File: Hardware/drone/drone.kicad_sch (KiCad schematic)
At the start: 11 parts, among them M1 Motor_DC, M2 Motor_DC, M3 Motor_DC, M4 Motor_DC, U1 ESP32-DEVKITC, U2 MPU6050 DevKit, U3 HW_611, U4 DRV8833, U5 DRV8833, U6 MT3608

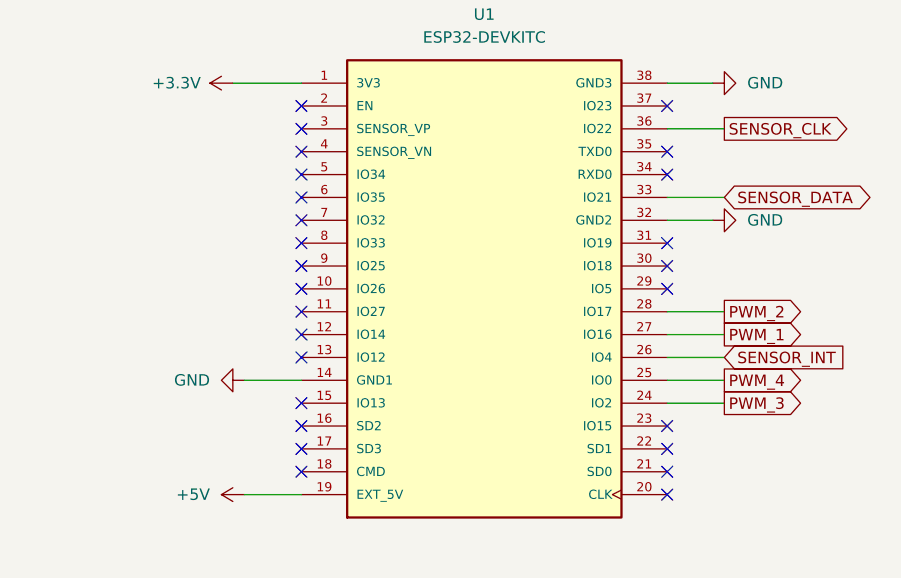
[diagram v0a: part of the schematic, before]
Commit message: PCB design v1.0
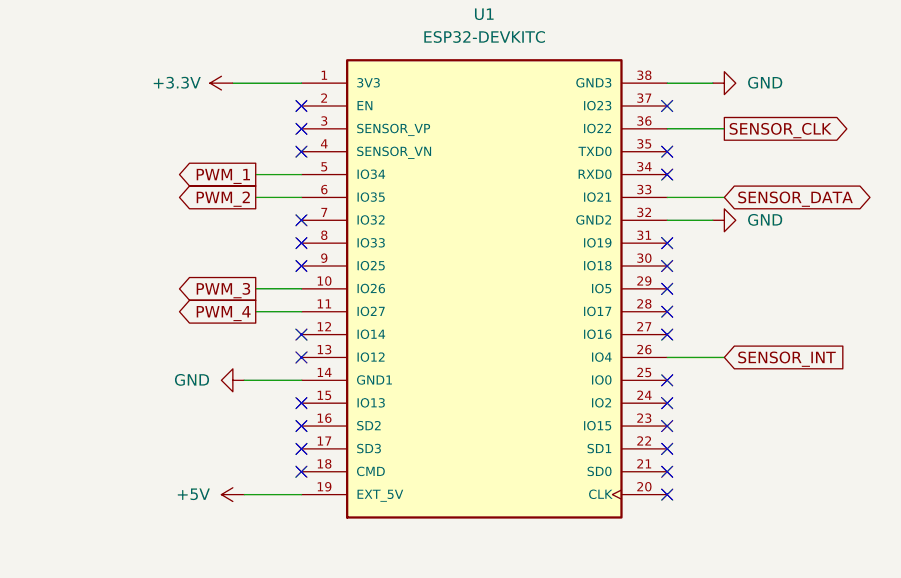
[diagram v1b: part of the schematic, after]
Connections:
- net PWM_1: now also U1.5 (IO34); no longer U1.27 (IO16)
- net PWM_2: now also U1.6 (IO35); no longer U1.28 (IO17)
- net PWM_3: now also U1.10 (IO26); no longer U1.24 (IO2)
- net PWM_4: now also U1.11 (IO27); no longer U1.25 (IO0)
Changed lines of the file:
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@@
+	)
+	(no_connect
+		(at 215.9 121.92)
 	)
 	(no_connect
@@
 	)
 	(no_connect
+		(at 215.9 119.38)
+	)
+	(no_connect
 		(at 128.27 48.26)
 	)
@@
 	)
 	(no_connect
-		(at 175.26 99.06)
-	)
-	(no_connect
 		(at 175.26 104.14)
 	)
 	(no_connect
-		(at 175.26 111.76)
-	)
-	(no_connect
 		(at 67.31 44.45)
 	)
 	(no_connect
+		(at 215.9 111.76)
+	)
+	(no_connect
 		(at 215.9 88.9)
 	)
@@
 	)
 	(no_connect
-		(at 175.26 109.22)
-	)
-	(no_connect
 		(at 175.26 93.98)
 	)
@@
 	)
 	(no_connect
-		(at 175.26 96.52)
+		(at 215.9 114.3)
 	)
 	(no_connect
@@
 	(wire
 		(pts
-			(xy 215.9 119.38) (xy 222.25 119.38)
+			(xy 170.18 99.06) (xy 175.26 99.06)
 		)
 		(stroke
@@
 	(wire
 		(pts
-			(xy 215.9 111.76) (xy 222.25 111.76)
+			(xy 170.18 96.52) (xy 175.26 96.52)
 		)
 		(stroke
@@
 	(wire
 		(pts
+			(xy 170.18 111.76) (xy 175.26 111.76)
+		)
+		(stroke
+			(width 0)
+			(type default)
+		)
+	)
+	(wire
+		(pts
 			(xy 215.9 86.36) (xy 220.98 86.36)
 		)
@@
 	(wire
 		(pts
+			(xy 170.18 109.22) (xy 175.26 109.22)
+		)
+		(stroke
+			(width 0)
+			(type default)
+		)
+	)
+	(wire
+		(pts
 			(xy 67.31 36.83) (xy 72.39 36.83)
 		)
@@
 	(wire
 		(pts
-			(xy 215.9 121.92) (xy 222.25 121.92)
-		)
-		(stroke
-			(width 0)
-			(type default)
-		)
-	)
-	(wire
-		(pts
-			(xy 215.9 114.3) (xy 222.25 114.3)
-		)
-		(stroke
-			(width 0)
-			(type default)
-		)
-	)
-	(wire
-		(pts
 			(xy 168.91 132.08) (xy 175.26 132.08)
 		)
@@
 		)
 	)
+	(global_label "PWM_4"
+		(shape output)
+		(at 170.18 111.76 180)
+		(fields_autoplaced yes)
+		(effects
+			(font
+				(size 1.27 1.27)
+			)
+			(justify right)
+		)
+		(property "Intersheetrefs" "${INTERSHEET_REFS}"
+			(at 160.8449 111.76 0)
+			(effects
+				(font
+					(size 1.27 1.27)
+				)
+				(justify right)
+				(hide yes)
+			)
+		)
+	)
 	(global_label "PWM_3"
 		(shape output)
-		(at 222.25 121.92 0)
-		(fields_autoplaced yes)
-		(effects
-			(font
-				(size 1.27 1.27)
-			)
-			(justify left)
-		)
-		(property "Intersheetrefs" "${INTERSHEET_REFS}"
-			(at 231.5851 121.92 0)
-			(effects
-				(font
-					(size 1.27 1.27)
-				)
-				(justify left)
+		(at 170.18 109.22 180)
+		(fields_autoplaced yes)
+		(effects
+			(font
+				(size 1.27 1.27)
+			)
+			(justify right)
+		)
+		(property "Intersheetrefs" "${INTERSHEET_REFS}"
+			(at 160.8449 109.22 0)
+			(effects
+				(font
+					(size 1.27 1.27)
+				)
+				(justify right)
 				(hide yes)
 			)
@@
 				)
 				(justify left)
+				(hide yes)
+			)
+		)
+	)
+	(global_label "PWM_2"
+		(shape output)
+		(at 170.18 99.06 180)
+		(fields_autoplaced yes)
+		(effects
+			(font
+				(size 1.27 1.27)
+			)
+			(justify right)
+		)
+		(property "Intersheetrefs" "${INTERSHEET_REFS}"
+			(at 160.8449 99.06 0)
+			(effects
+				(font
+					(size 1.27 1.27)
+				)
+				(justify right)
 				(hide yes)
 			)
@@
 		)
 	)
-	(global_label "PWM_2"
-		(shape output)
-		(at 222.25 111.76 0)
-		(fields_autoplaced yes)
-		(effects
-			(font
-				(size 1.27 1.27)
-			)
-			(justify left)
-		)
-		(property "Intersheetrefs" "${INTERSHEET_REFS}"
-			(at 231.5851 111.76 0)
-			(effects
-				(font
-					(size 1.27 1.27)
-				)
-				(justify left)
+	(global_label "PWM_1"
+		(shape output)
+		(at 170.18 96.52 180)
+		(fields_autoplaced yes)
+		(effects
+			(font
+				(size 1.27 1.27)
+			)
+			(justify right)
+		)
+		(property "Intersheetrefs" "${INTERSHEET_REFS}"
+			(at 160.8449 96.52 0)
+			(effects
+				(font
+					(size 1.27 1.27)
+				)
+				(justify right)
 				(hide yes)
 			)
@@
 		)
 	)
-	(global_label "PWM_4"
-		(shape output)
-		(at 222.25 119.38 0)
-		(fields_autoplaced yes)
-		(effects
-			(font
-				(size 1.27 1.27)
-			)
-			(justify left)
-		)
-		(property "Intersheetrefs" "${INTERSHEET_REFS}"
-			(at 231.5851 119.38 0)
-			(effects
-				(font
-					(size 1.27 1.27)
-				)
-				(justify left)
-				(hide yes)
-			)
-		)
-	)
 	(global_label "SENSOR_INT"
 		(shape input)
@@
 			(effects
 				(font
-					(size 1.27 1.27)
-				)
-				(justify left)
-				(hide yes)
-			)
-		)
-	)
-	(global_label "PWM_1"
-		(shape output)
-		(at 222.25 114.3 0)
-		(fields_autoplaced yes)
-		(effects
-			(font
-				(size 1.27 1.27)
-			)
-			(justify left)
-		)
-		(property "Intersheetrefs" "${INTERSHEET_REFS}"
-			(at 231.5851 114.3 0)
-			(effects
-				(font
